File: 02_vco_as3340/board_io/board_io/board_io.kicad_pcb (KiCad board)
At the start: 2 copper layers, 72.4 x 35.6 mm, 9 parts, among them J1 Header 1, J2 Header 2, SW2 SW_SPDT

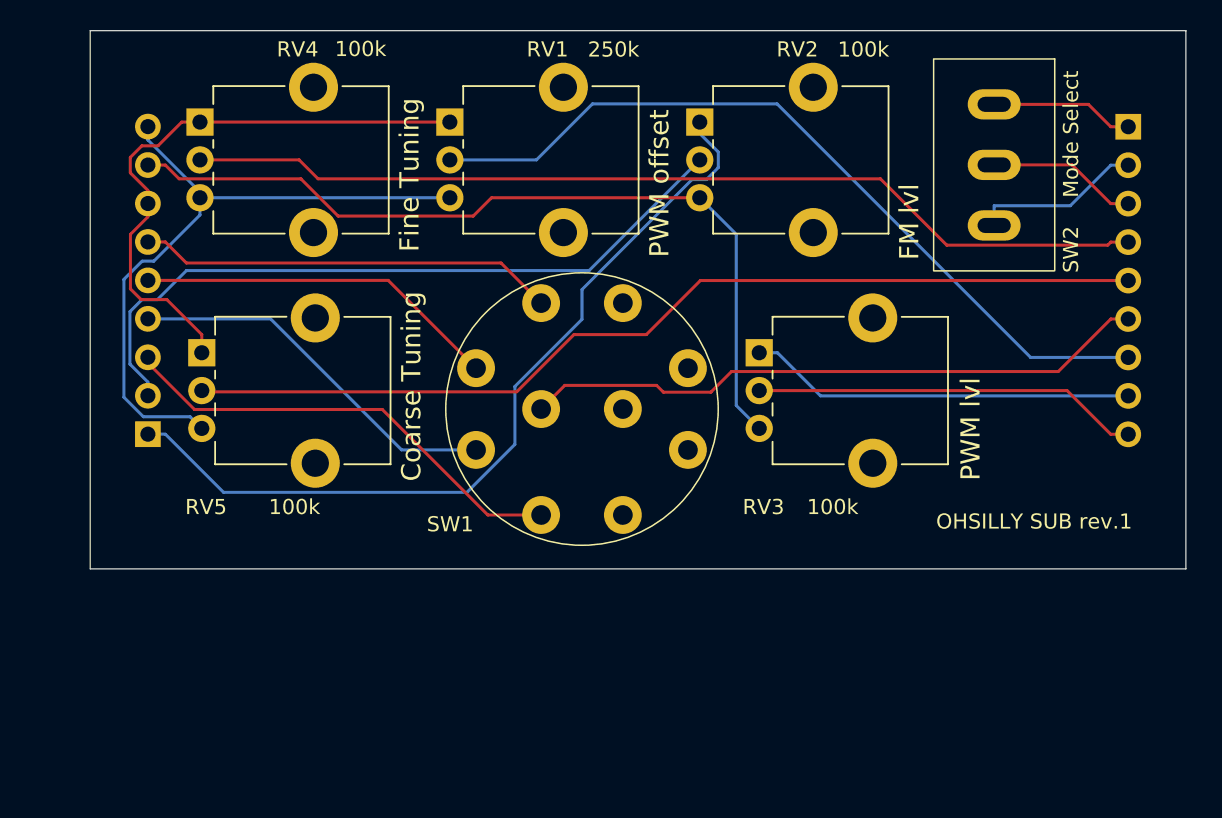
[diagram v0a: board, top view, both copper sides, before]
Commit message: routed everyting
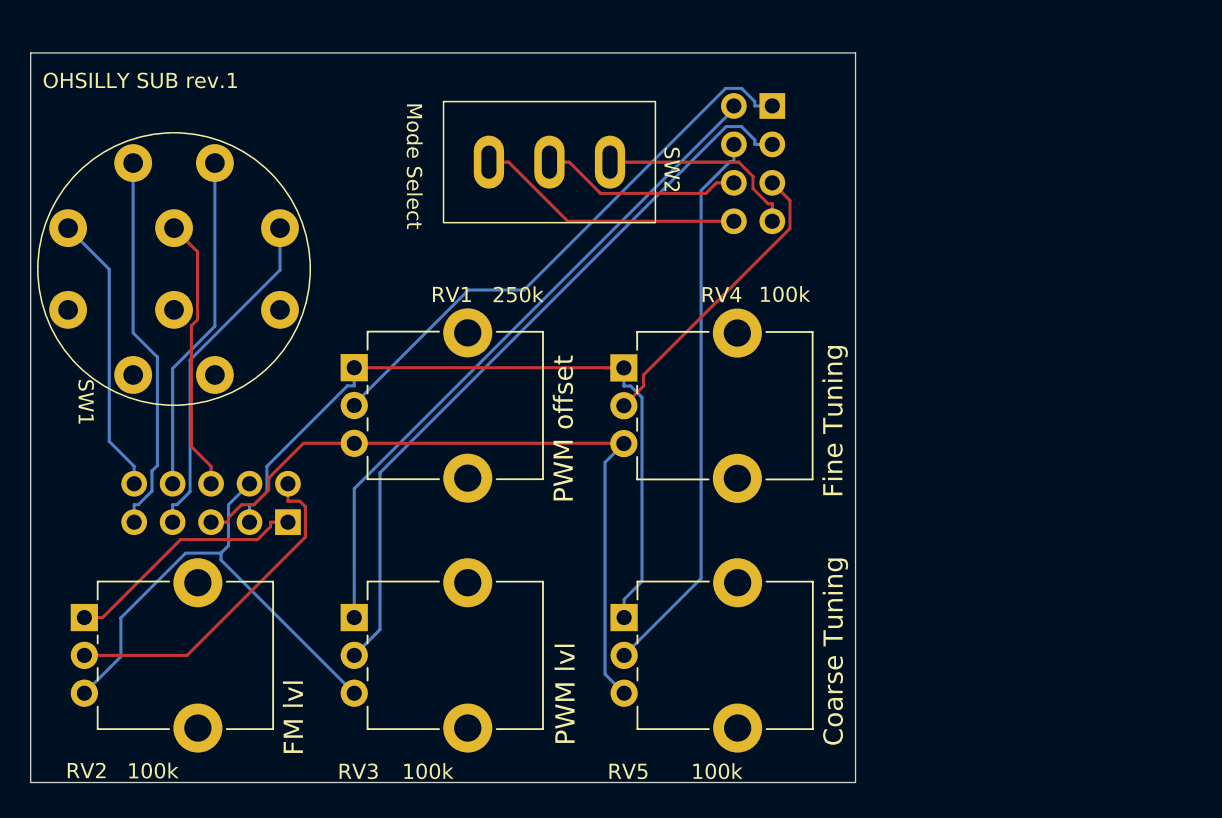
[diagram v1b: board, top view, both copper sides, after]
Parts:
- removed J1: Header 1, Connector_PinHeader_2.54mm:PinHeader_1x09_P2.54mm_Vertical
- removed J2: Header 2, Connector_PinHeader_2.54mm:PinHeader_1x09_P2.54mm_Vertical
- added J3: Header 1, Connector_PinHeader_2.54mm:PinHeader_2x05_P2.54mm_Vertical, B.Cu at (32.4, 49.3)
- added J4: Header 2, Connector_PinHeader_2.54mm:PinHeader_2x04_P2.54mm_Vertical, B.Cu at (64.4, 21.8)
- moved RV2 52.2 mm to (19.0, 55.6)
- moved RV5 32.9 mm to (54.6, 55.6)
- moved RV4 32.4 mm to (54.6, 39.1)
- moved RV3 32.0 mm to (36.8, 55.6)
- moved SW2 29.4 mm to (49.7, 25.5), turned to 0 degrees
- moved SW1 28.5 mm to (24.9, 32.6), turned to -90 degrees
- moved RV1 17.4 mm to (36.8, 39.1)
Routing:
- net Fine Tuning: track 63.7 -> 19.8 mm
- net FM CV Hot: track 55.1 -> 16.2 mm
- net Coarse Tuning: track 64.3 -> 36.9 mm
- net FM CV Levelled: track 47.8 -> 22.3 mm
- net Sync COM: track 41.6 -> 18.2 mm
- net PWM CV Levelled: track 25.6 -> 48.8 mm
- net GND: track 55.2 -> 32.6 mm
- net PWM CV Hot: track 25.6 -> 44.2 mm
- net PWM Offset: track 53.3 -> 37.0 mm
- net Hard Sync +: track 30.5 -> 18.7 mm
- net +12V: track 38.9 -> 49.1 mm
- net Mode LFO: track 9.47 -> 17.8 mm
- net Soft Sync: track 27.7 -> 22.5 mm
- net Mode COM: track 9.92 -> 13.3 mm
- net -12V: track 44.3 -> 47.6 mm
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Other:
- board size 72.4 x 35.6 mm -> 54.5 x 48.2 mm
